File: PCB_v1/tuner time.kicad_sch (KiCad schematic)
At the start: 2 parts, among them J1 Conn_01x03, U1 C1F 2

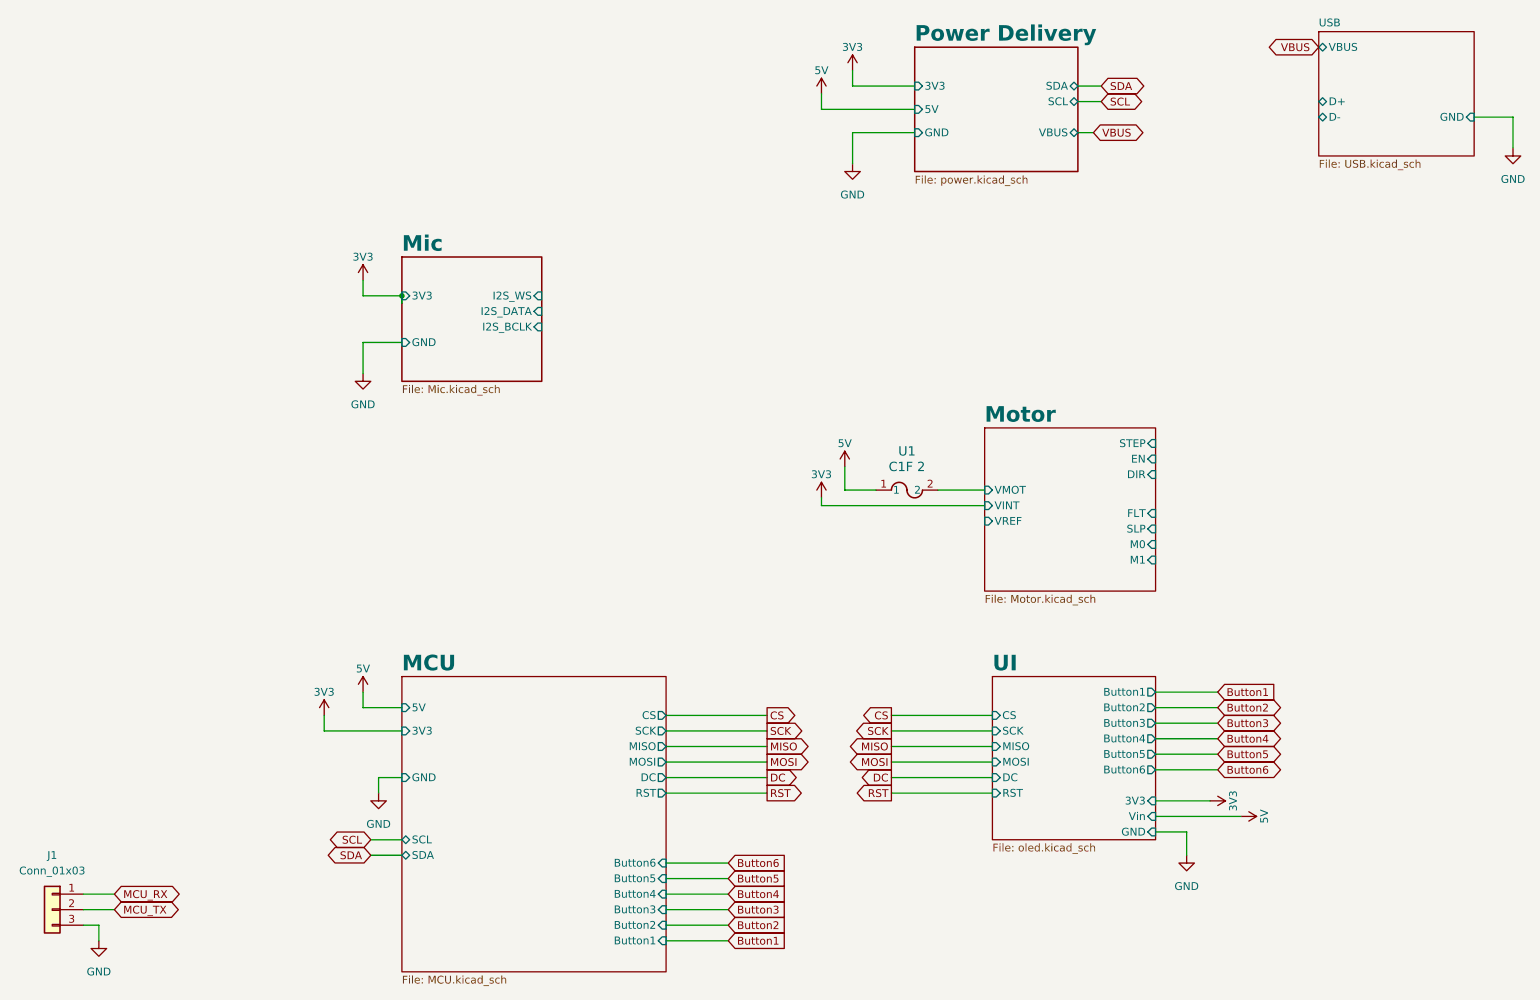
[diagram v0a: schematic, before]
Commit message: Initial placement draft
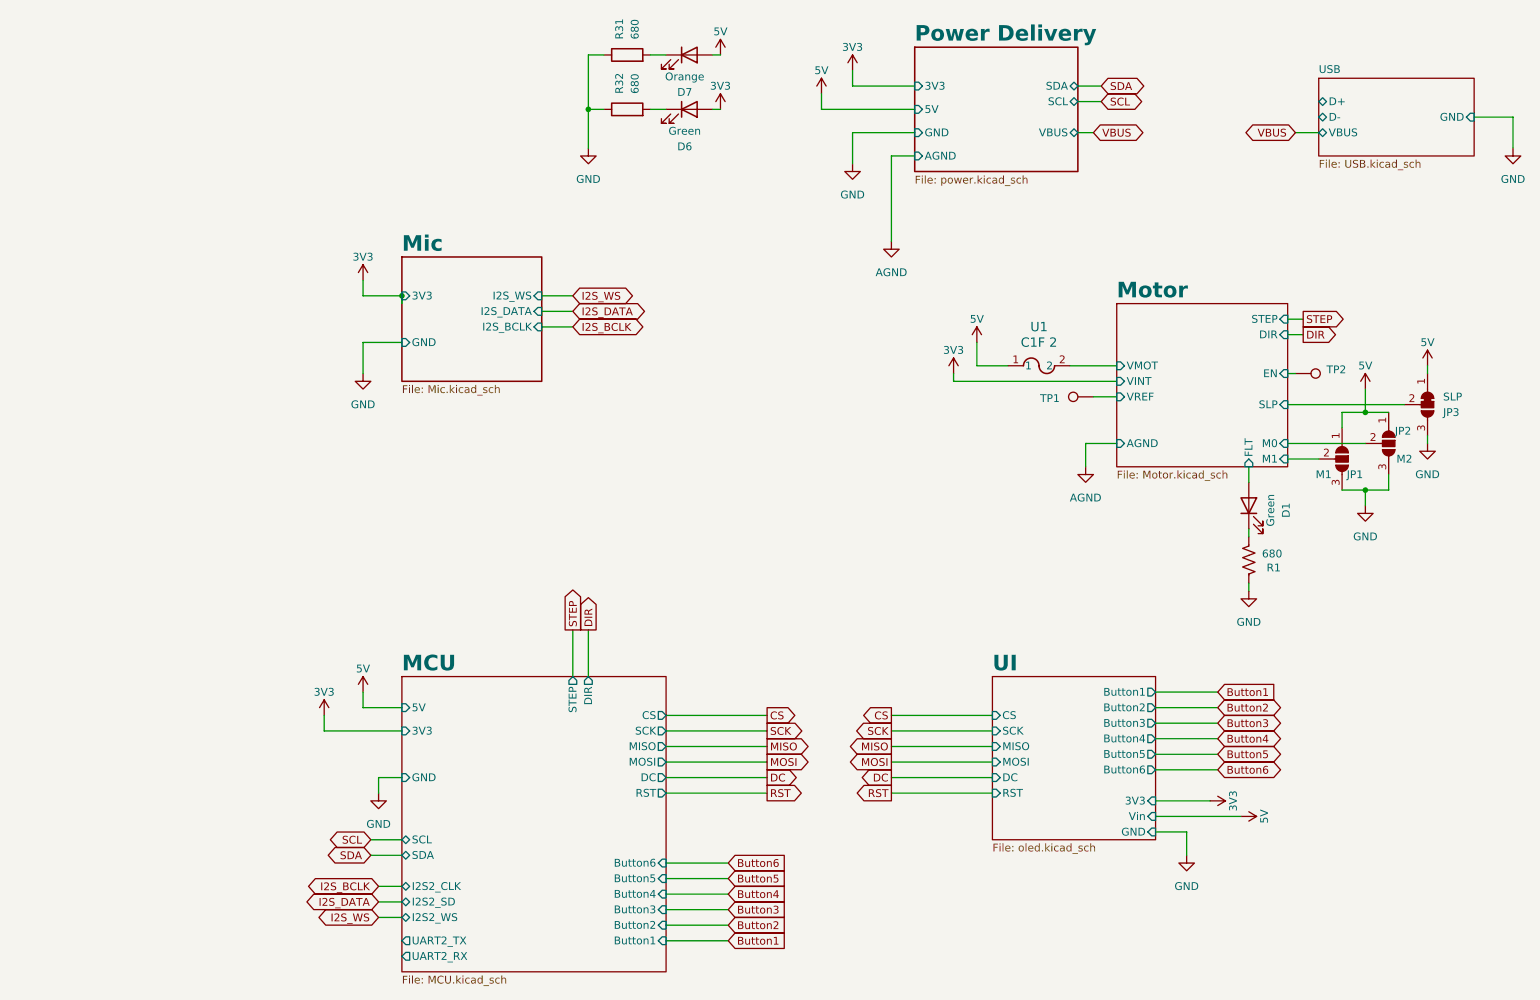
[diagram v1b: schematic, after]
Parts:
- removed J1: Conn_01x03, symbol Connector_Generic:Conn_01x03
- added D1, D6: Green, LED_SMD:LED_0805_2012Metric_Pad1.15x1.40mm_HandSolder, symbol Device:LED
- added D7: Orange, LED_SMD:LED_0805_2012Metric_Pad1.15x1.40mm_HandSolder, symbol Device:LED
- added JP1: M1, Jumper:SolderJumper-3_P1.3mm_Open_RoundedPad1.0x1.5mm, symbol Jumper:SolderJumper_3_Open
- added JP2: M2, Jumper:SolderJumper-3_P1.3mm_Open_RoundedPad1.0x1.5mm, symbol Jumper:SolderJumper_3_Open
- added JP3: SLP, Jumper:SolderJumper-3_P1.3mm_Bridged12_RoundedPad1.0x1.5mm, symbol Jumper:SolderJumper_3_Bridged12
- added R1: 680, Resistor_SMD:R_0805_2012Metric, symbol Device:R_US
- added R31, R32: 680, Resistor_SMD:R_0805_2012Metric, symbol Device:R
- added TP1, TP2: ~, TestPoint:TestPoint_THTPad_D1.0mm_Drill0.5mm, symbol Connector:TestPoint
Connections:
- net 3V3: now also D6.2 (A)
- net 5V: now also D7.2 (A), JP1.1 (A), JP2.1 (A), JP3.1 (A)
- net GND: now also JP1.3 (B), JP2.3 (B), JP3.3 (B), R1.2, R31.1, R32.1
- net Motor/EN: now also TP2.1
- net Motor/FLT: now also D1.2 (A)
- net Motor/M0: now also JP2.2 (C)
- net Motor/M1: now also JP1.2 (C)
- net Motor/SLP: now also JP3.2 (C)
- net Motor/VREF: now also TP1.1
- new net: D7.1 (K), R31.2
- new net: D6.1 (K), R32.2
- new net: D1.1 (K), R1.1
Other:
- sheet MCU ports: added DIR, I2S2_CLK, I2S2_SD, I2S2_WS, STEP, UART2_RX, UART2_TX; removed none
- sheet Motor ports: added AGND; removed none
- sheet Power Delivery ports: added AGND; removed none
- moved on the sheet: U1
